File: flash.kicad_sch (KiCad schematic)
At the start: 2 parts, among them U2 SST26VF016BEUI-104I/SN

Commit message: #1 Use new central library KiCad-Lib
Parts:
- U2: symbol Project_Library:Microchip Technology SST26VF016BEUI-104I/SN -> #IC:Microchip Technology SST26VF016BEUI-104I/SN; now in the parts list
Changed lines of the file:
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@@
     (effects (font (size 1 1)) (justify right))
   )
-  (symbol (lib_id "Project_Library:Microchip Technology SST26VF016BEUI-104I/SN") (at 71.755 34.925 0) (unit 1)
-    (in_bom no) (on_board yes) (dnp yes) (fields_autoplaced)
+  (symbol (lib_id "#IC:Microchip Technology SST26VF016BEUI-104I/SN") (at 71.755 34.925 0) (unit 1)
+    (in_bom yes) (on_board yes) (dnp yes) (fields_autoplaced)
     (property "Reference" "U2" (at 81.28 33.6549 0)
       (effects (font (size 1 1)) (justify left))
@@
       (effects (font (size 1.27 1.27)) hide)
     )
-    (property "Datasheet" "http://ww1.microchip.com/downloads/en/DeviceDoc/20005045C.pdf" (at 71.755 57.785 0)
+    (property "Datasheet" "${KIPRJMOD}/KiCad-Lib/#IC.doc/Microchip Technology SST26VF016BEUI-104ISN.pdf" (at 71.755 57.785 0)
       (effects (font (size 1.27 1.27)) hide)
     )

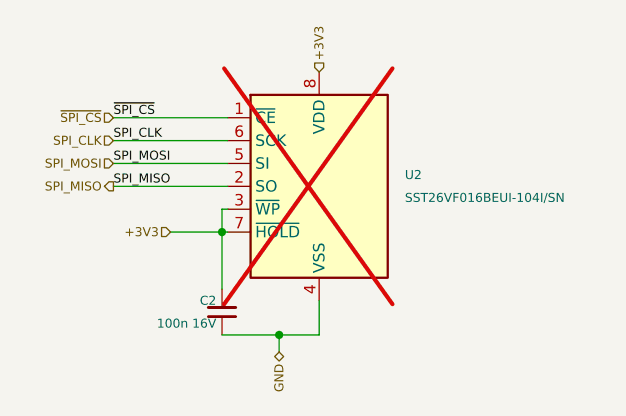
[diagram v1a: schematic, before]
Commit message: WIP
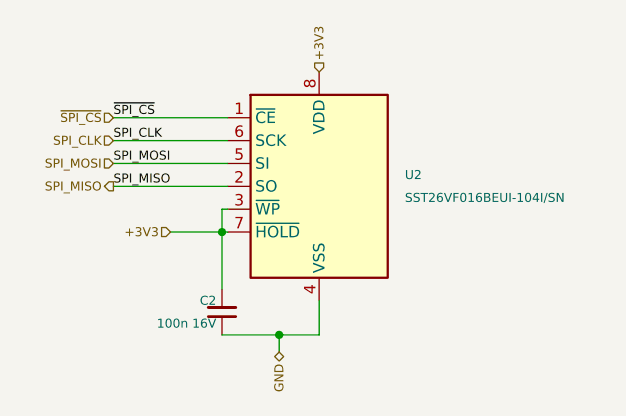
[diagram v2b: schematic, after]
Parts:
- U2: now fitted; now left out of the parts list
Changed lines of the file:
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@@
   )
   (symbol (lib_id "#IC:Microchip Technology SST26VF016BEUI-104I/SN") (at 71.755 34.925 0) (unit 1)
-    (in_bom yes) (on_board yes) (dnp yes) (fields_autoplaced)
+    (in_bom no) (on_board yes) (dnp no) (fields_autoplaced)
     (property "Reference" "U2" (at 81.28 33.6549 0)
       (effects (font (size 1 1)) (justify left))
@@
         )
         (path "/e63e39d7-6ac0-4ffd-8aa3-1841a4541b55/0d09f1c5-80ef-4ecd-bc99-7e5b757caf07"
-          (reference "U501") (unit 1)
+          (reference "U301") (unit 1)
         )
       )
@@
       (project "stm32f4_uno"
         (path "/e63e39d7-6ac0-4ffd-8aa3-1841a4541b55/0d09f1c5-80ef-4ecd-bc99-7e5b757caf07"
-          (reference "C501") (unit 1)
+          (reference "C301") (unit 1)
         )
       )

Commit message: #2 Add silkscreen texts
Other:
- company: (none) -> easy-smart solution GmbH
- title: (none) -> STM32F4 Uno
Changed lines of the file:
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@@
 (kicad_sch (version 20230121) (generator eeschema)
   (paper "A4")
+  (title_block
+    (title "STM32F4 Uno")
+    (date "2023-10-02")
+    (rev "1.0.x-dev")
+    (company "easy-smart solution GmbH")
+  )
   (junction (at 67.31 51.435) (diameter 0) (color 0 0 0 0)
   )
